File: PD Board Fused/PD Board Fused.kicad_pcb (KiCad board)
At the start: 4 copper layers, 97 x 32.5 mm, 19 parts, among them J1 Conn_02x02_Odd_Even, P1 2604-1102, P2 2604-1102, P3 2604-1102, P4 2604-1102, P5 2604-1102, P6 2604-1102, P7 2604-1102, P8 2604-1102, P9 2604-1102, U1 MCP1792T-3302H/CB

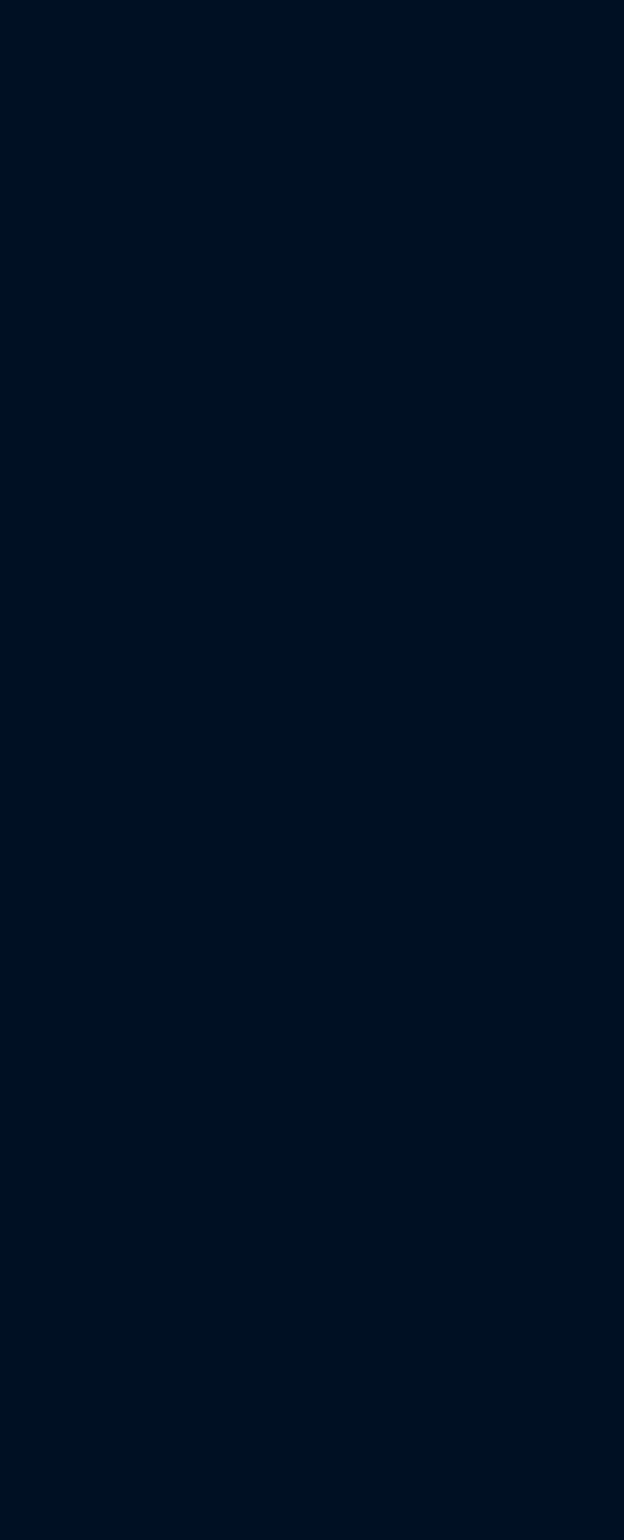
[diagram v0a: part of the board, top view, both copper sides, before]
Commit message: started fused board
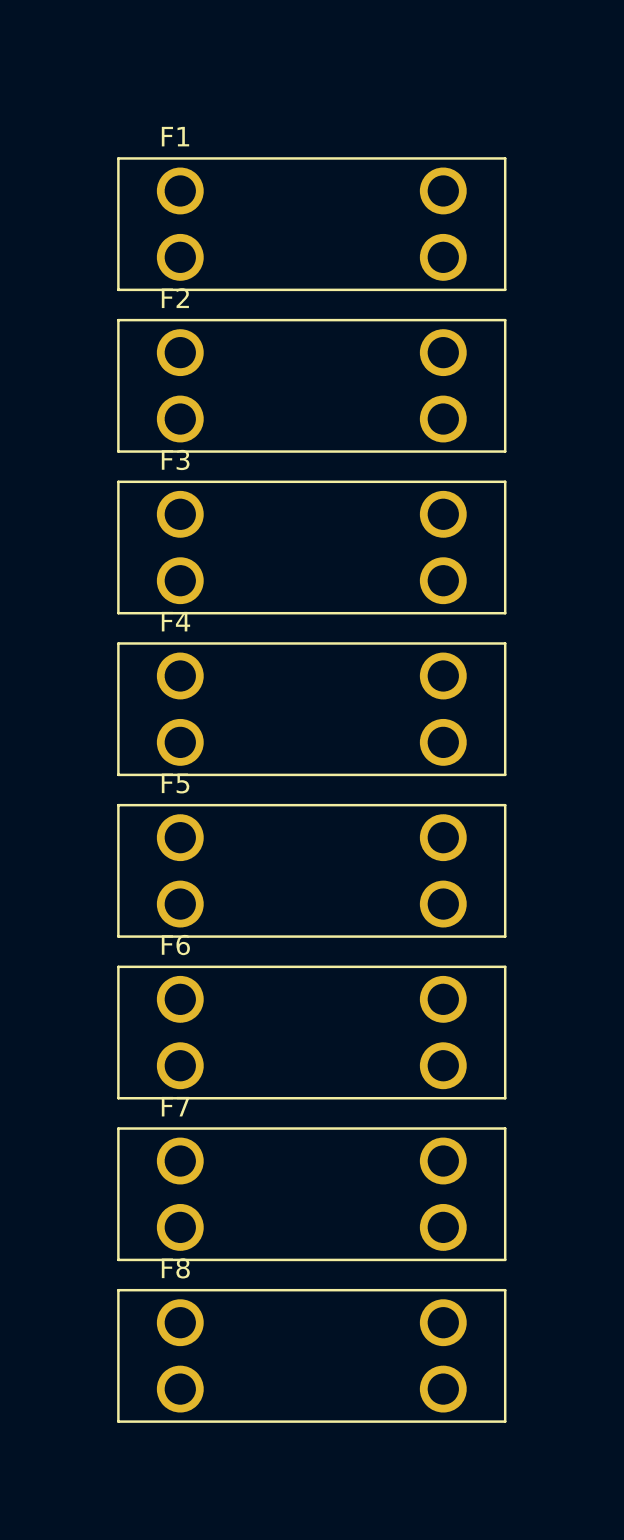
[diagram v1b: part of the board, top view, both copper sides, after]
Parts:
- added F1: 3557-2, Customconnectors:FUSE_3557-2, F.Cu at (55.9, 88.4)
- added F2: 3557-2, Customconnectors:FUSE_3557-2, F.Cu at (55.9, 96.7)
- added F3: 3557-2, Customconnectors:FUSE_3557-2, F.Cu at (55.9, 105.0)
- added F4: 3557-2, Customconnectors:FUSE_3557-2, F.Cu at (55.9, 113.3)
- added F5: 3557-2, Customconnectors:FUSE_3557-2, F.Cu at (55.9, 121.5)
- added F6: 3557-2, Customconnectors:FUSE_3557-2, F.Cu at (55.9, 129.8)
- added F7: 3557-2, Customconnectors:FUSE_3557-2, F.Cu at (55.9, 138.1)
- added F8: 3557-2, Customconnectors:FUSE_3557-2, F.Cu at (55.9, 146.4)
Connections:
- P1 pad 3: +20V -> Net-(P1-2.1)
- P1 pad 4: +20V -> Net-(P1-2.1)
- P2 pad 3: +20V -> Net-(P2-2.1)
- P2 pad 4: +20V -> Net-(P2-2.1)
- P3 pad 3: +20V -> Net-(P3-2.1)
- P3 pad 4: +20V -> Net-(P3-2.1)
- P4 pad 3: +20V -> Net-(P4-2.1)
- P4 pad 4: +20V -> Net-(P4-2.1)
- P5 pad 3: +20V -> Net-(P5-2.1)
- P5 pad 4: +20V -> Net-(P5-2.1)
- P6 pad 3: +20V -> Net-(P6-2.1)
- P6 pad 4: +20V -> Net-(P6-2.1)
- P7 pad 3: +20V -> Net-(P7-2.1)
- P7 pad 4: +20V -> Net-(P7-2.1)
- P8 pad 3: +20V -> Net-(P8-2.1)
- P8 pad 4: +20V -> Net-(P8-2.1)
